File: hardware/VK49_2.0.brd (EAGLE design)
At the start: 35 x 35 mm, 60 parts, among them IC1 ATSAMD21G18A-MU, IC2 SPI_FLASH, IC3 MCP73831T-2ACI, IC4 MAX98357AETE+, IC5 DS3231MZ+, IC6 STM6519, J1 USB-C, Q1 LGE2305, Q2 LGE2305, Q3 2N3904, SW1 KSC341J-LFS, SW2 KSR221G-LFS, Y1 32.768 kHz

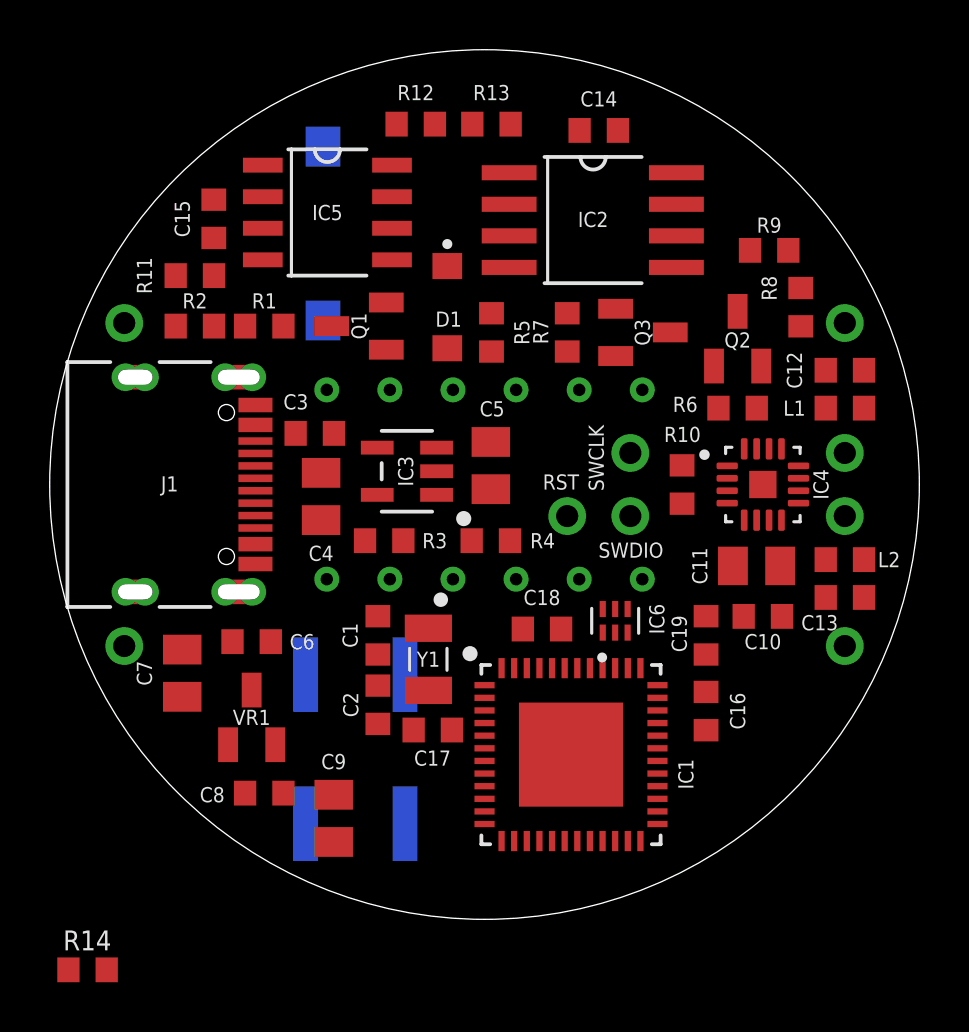
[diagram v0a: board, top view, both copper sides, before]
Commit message: 2.0 board in progress
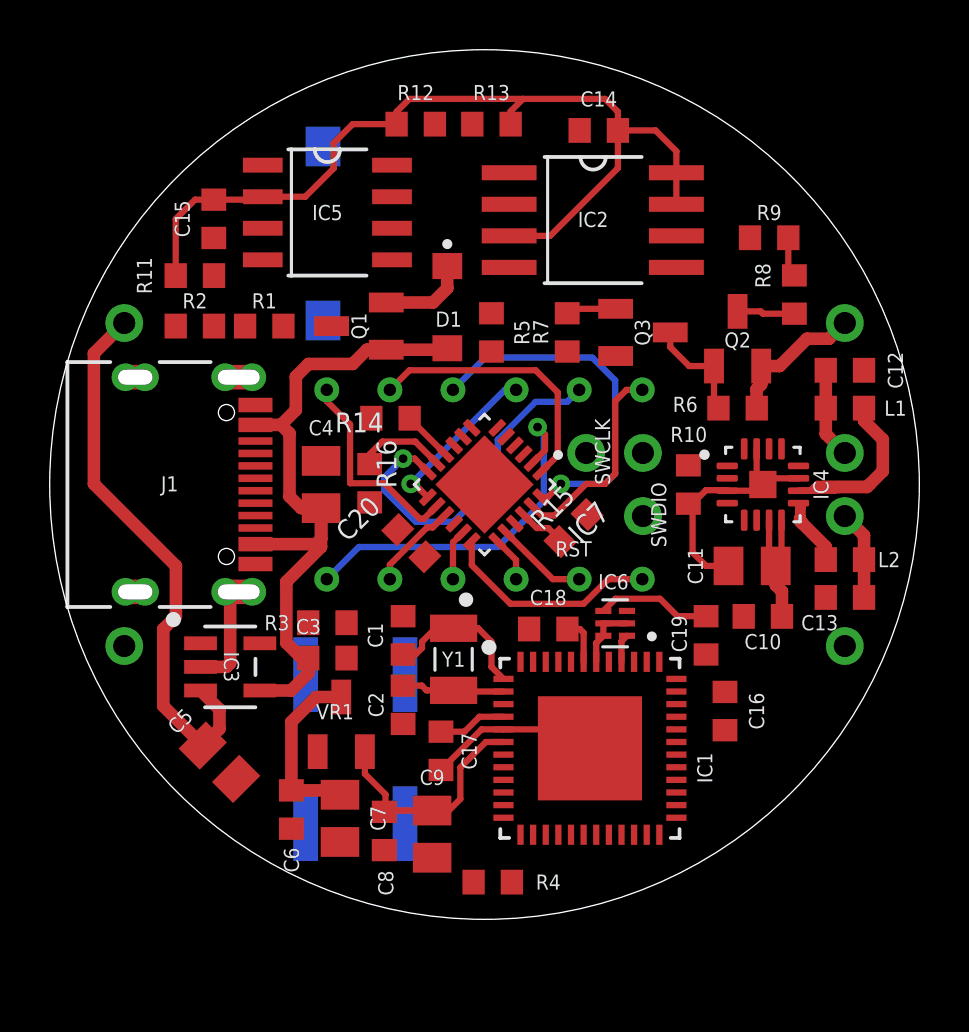
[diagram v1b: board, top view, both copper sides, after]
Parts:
- added C20: 100n, BASTL_CAPACITORS:CAPACITOR0603
- added IC7: AS1115-BQFT, BASTL_ICS:QFN50P400X400X65-25N
- added R15, R16: 4k7, BASTL_RESISTORS:RESISTOR0603
- R14: value 100 -> 10k
- moved R14 25.3 mm to (13.7, 20.2), turned to 180 degrees
- moved C5 16.2 mm to (6.83, 6.32), turned to 315 degrees
- moved R4 13.7 mm to (17.8, 1.50), turned to 180 degrees
- moved IC3 10.6 mm to (7.26, 10.2), turned to 0 degrees
- moved C3 9.06 mm to (11.2, 10.5)
- moved C7 8.63 mm to (11.7, 4.06), turned to 270 degrees
- moved C6 6.94 mm to (9.73, 4.42), turned to 90 degrees
- moved C8 5.06 mm to (13.5, 3.56), turned to 90 degrees
- moved R3 4.02 mm to (11.2, 11.9), turned to 180 degrees
- moved C9 4.01 mm to (15.4, 3.43)
- moved VR1 3.62 mm to (11.7, 7.85)
- moved JP9 2.65 mm to (21.6, 18.8)
- moved C1 1.02 mm to (14.2, 11.4)
- moved C2 1.02 mm to (14.2, 8.64)
- moved Y1 1.02 mm to (16.3, 10.5)
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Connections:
- new net N$12: DISPLAY1.12, IC7.23
- new net N$13: DISPLAY1.9, IC7.24
- new net N$14: DISPLAY1.8, IC7.1
- new net N$15: DISPLAY1.6, IC7.2
- new net N$16: DISPLAY1.11, IC7.12
- new net N$17: DISPLAY1.7, IC7.14
- new net N$18: DISPLAY1.4, IC7.17
- new net N$19: DISPLAY1.2, IC7.20
- new net N$20: DISPLAY1.1, IC7.18
- new net N$21: DISPLAY1.10, IC7.13
- new net N$22: DISPLAY1.5, IC7.15
- new net N$23: DISPLAY1.3, IC7.19
- new net N$3: IC7.10, R14.1
- net ENABLED: now also R7.1
- net GND: now also C20.1, IC7.3
- net SCL: now also IC7.11, R16.1
- net SDA: now also IC7.22, R15.1
- net VDD: now also C20.2, IC7.16, R14.2, R15.2, R16.2; no longer R7.1
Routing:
- net VDD: track 0.00 -> 51.1 mm
- net VBAT: track 0.00 -> 28.4 mm
- net VBUS: track 0.00 -> 28.2 mm
- net GND: track 0.00 -> 23.9 mm
- net UNREG: track 0.00 -> 16.8 mm
- net N$15: track 0.00 -> 14.9 mm, vias 0 -> 1
- net N$13: track 0.00 -> 14.6 mm, vias 0 -> 1
- net N$16: track 0.00 -> 14.3 mm, vias 0 -> 1
- net N$8: track 0.00 -> 11.1 mm
- net N$14: track 0.00 -> 10.9 mm
- net N$20: track 0.00 -> 8.88 mm
- net N$17: track 0.00 -> 8.43 mm
- net N$12: track 0.00 -> 8.38 mm
- net N$21: track 0.00 -> 6.74 mm, vias 0 -> 1
- net N$1: track 0.00 -> 6.06 mm
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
